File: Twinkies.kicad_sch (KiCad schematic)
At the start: 0 parts

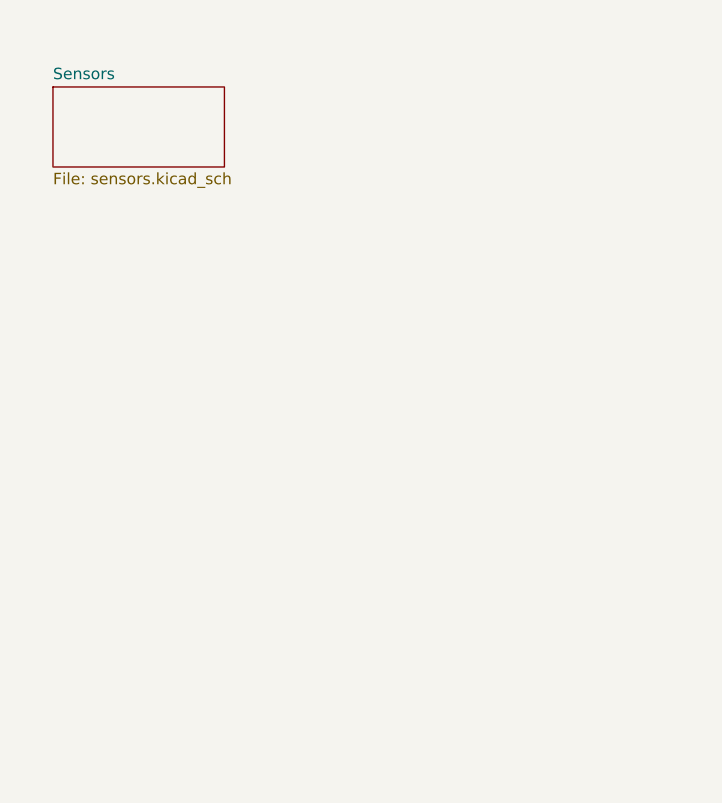
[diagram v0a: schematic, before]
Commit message: 3.4
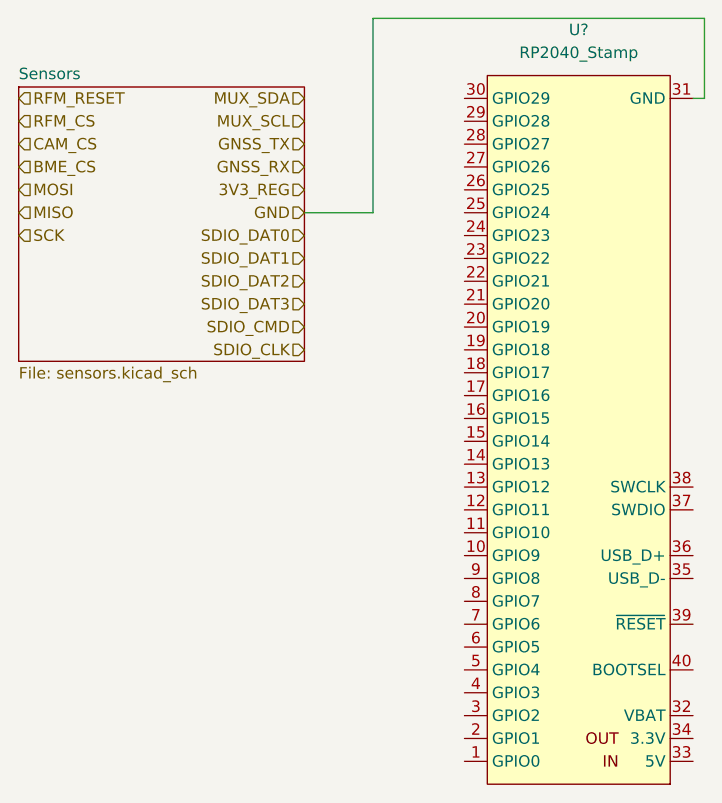
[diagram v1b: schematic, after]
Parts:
- added U?: RP2040_Stamp, RP2040_Stamp:RP2040_Stamp_SMD, symbol RP2040_Stamp:RP2040_Stamp
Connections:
- new net GND: U?.31 (GND)

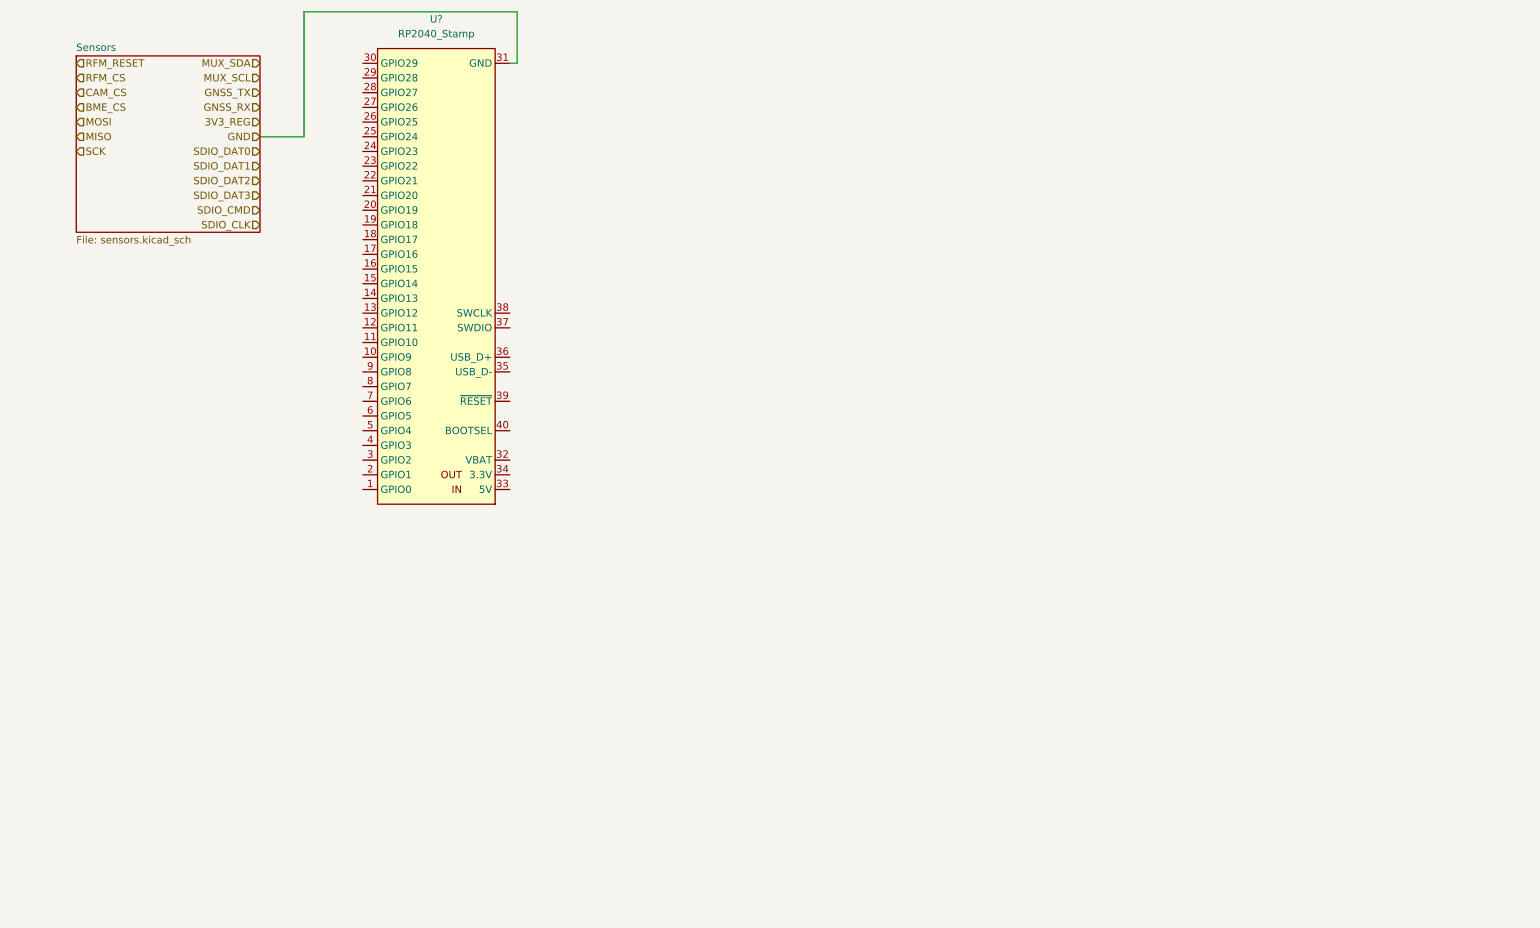
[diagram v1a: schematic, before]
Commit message: 3/6
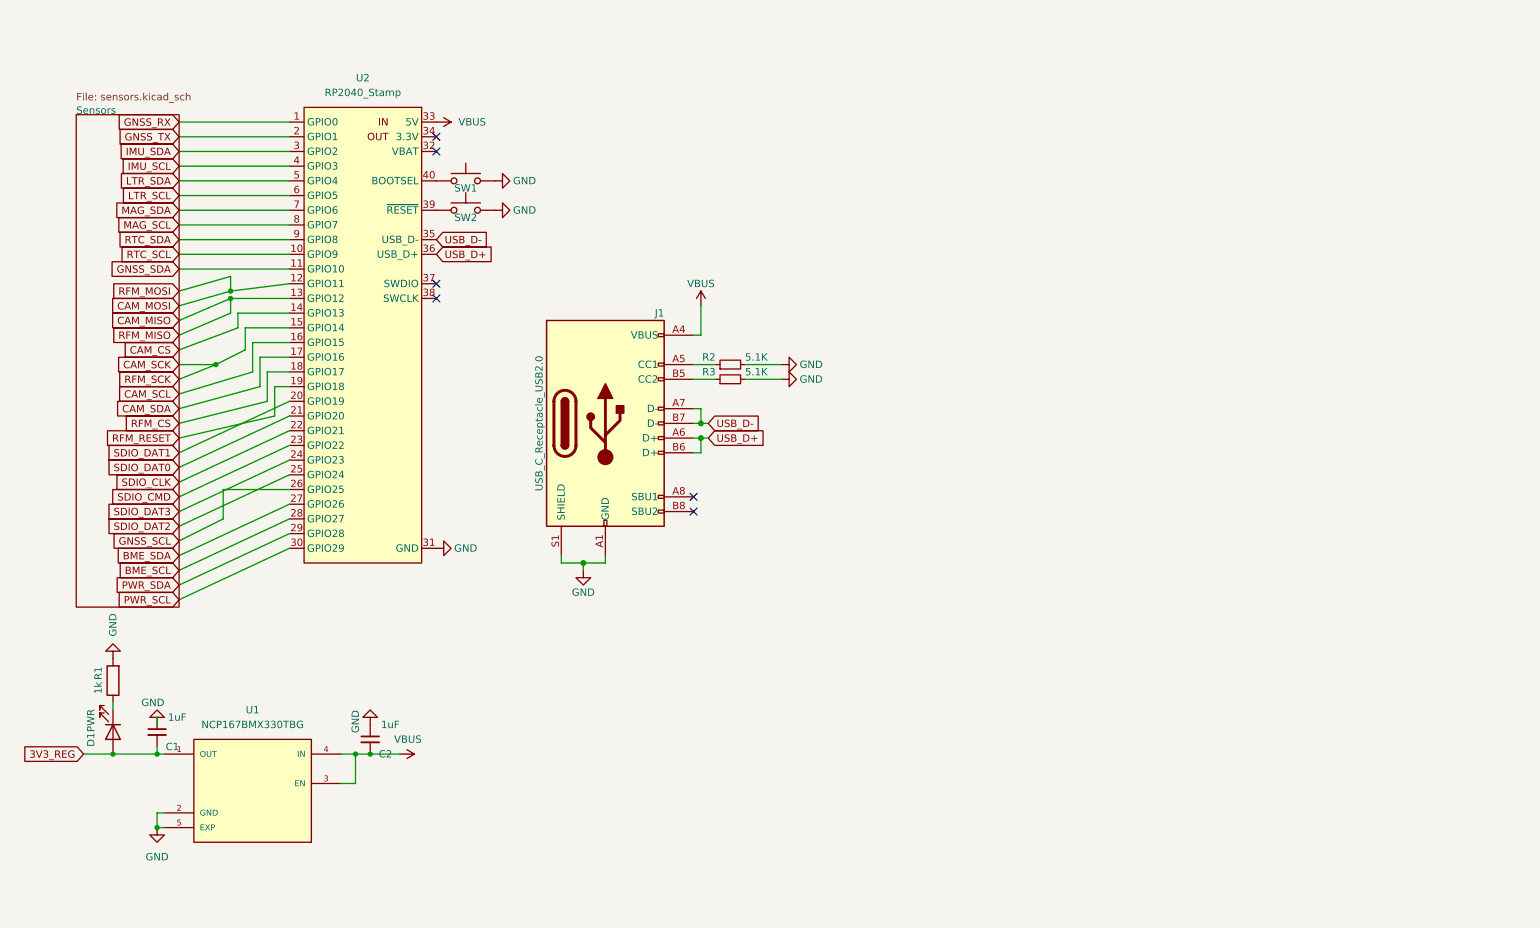
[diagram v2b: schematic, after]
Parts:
- added C1, C2: 1uF, Capacitor_SMD:C_0603_1608Metric, symbol Device:C_Small
- added D1: PWR, LED_SMD:LED_0603_1608Metric, symbol Device:LED
- added J1: USB_C_Receptacle_USB2.0, Connector_USB:USB_C_Receptacle_XKB_U262-16XN-4BVC11, symbol Connector:USB_C_Receptacle_USB2.0
- added R1: 1k, Resistor_SMD:R_0603_1608Metric, symbol Device:R
- added R2, R3: 5.1K, Resistor_SMD:R_0603_1608Metric, symbol Device:R_Small
- added SW1, SW2: RESET, Button_Switch_SMD:SW_Push_SPST_NO_Alps_SKRK, symbol Switch:SW_Push
- added U1: NCP167BMX330TBG, REG_NCP167BMX330TBG, symbol NCP167BMX330TBG:NCP167BMX330TBG
- gave numbers to parts that had none: 1
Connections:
- net 3V3_REG: now also C1.2, D1.2 (A), U1.1 (OUT)
- net CAM_CS: now also U2.14 (GPIO13)
- net GND: now also C1.1, C2.1, J1.A1 (GND), J1.A12 (GND), J1.B1 (GND), J1.B12 (GND), J1.S1 (SHIELD), R1.2, R2.2, R3.2, SW1.2, SW2.2, U1.2 (GND), U1.5 (EXP)
- net GNSS_RX: now also U2.1 (GPIO0)
- net GNSS_TX: now also U2.2 (GPIO1)
- net RFM_CS: now also U2.18 (GPIO17)
- net RFM_RESET: now also U2.19 (GPIO18)
- net SDIO_CLK: now also U2.22 (GPIO21)
- net SDIO_CMD: now also U2.23 (GPIO22)
- net SDIO_DAT0: now also U2.21 (GPIO20)
- net SDIO_DAT1: now also U2.20 (GPIO19)
- net SDIO_DAT2: now also U2.25 (GPIO24)
- net SDIO_DAT3: now also U2.24 (GPIO23)
- net RTC_SCL: now reaches U2.10 (GPIO9)
- net GNSS_SDA: now reaches U2.11 (GPIO10)
- net CAM_MOSI: now reaches U2.12 (GPIO11)
- net CAM_MISO: now reaches U2.13 (GPIO12)
- net CAM_SCK: now reaches U2.15 (GPIO14)
- net CAM_SCL: now reaches U2.16 (GPIO15)
- net CAM_SDA: now reaches U2.17 (GPIO16)
- net GNSS_SCL: now reaches U2.26 (GPIO25)
- net BME_SDA: now reaches U2.27 (GPIO26)
- net BME_SCL: now reaches U2.28 (GPIO27)
- net PWR_SDA: now reaches U2.29 (GPIO28)
- net IMU_SDA: now reaches U2.3 (GPIO2)
- net PWR_SCL: now reaches U2.30 (GPIO29)
- net VBUS: now reaches U2.33 (5V)
- net VBUS: now also C2.2, J1.A4 (VBUS), J1.A9 (VBUS), J1.B4 (VBUS), J1.B9 (VBUS), U1.3 (EN), U1.4 (IN)
- net USB_D-: now reaches U2.35 (USB_D-)
- net USB_D-: now also J1.A7 (D-), J1.B7 (D-)
- net USB_D+: now reaches U2.36 (USB_D+)
- net USB_D+: now also J1.A6 (D+), J1.B6 (D+)
- net at U2.39 (~{RESET}): now also SW2.1
- net IMU_SCL: now reaches U2.4 (GPIO3)
- net at U2.40 (BOOTSEL): now also SW1.1
- net LTR_SDA: now reaches U2.5 (GPIO4)
- net LTR_SCL: now reaches U2.6 (GPIO5)
- net MAG_SDA: now reaches U2.7 (GPIO6)
- net MAG_SCL: now reaches U2.8 (GPIO7)
- net RTC_SDA: now reaches U2.9 (GPIO8)
- new net: J1.B5 (CC2), R3.1
- new net: J1.A5 (CC1), R2.1
- new net: D1.1 (K), R1.1
- no-connect marks 0 -> 6
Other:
- title: Sensor Board -> RP2040 Stamp
- moved on the sheet: U2

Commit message: pdu design
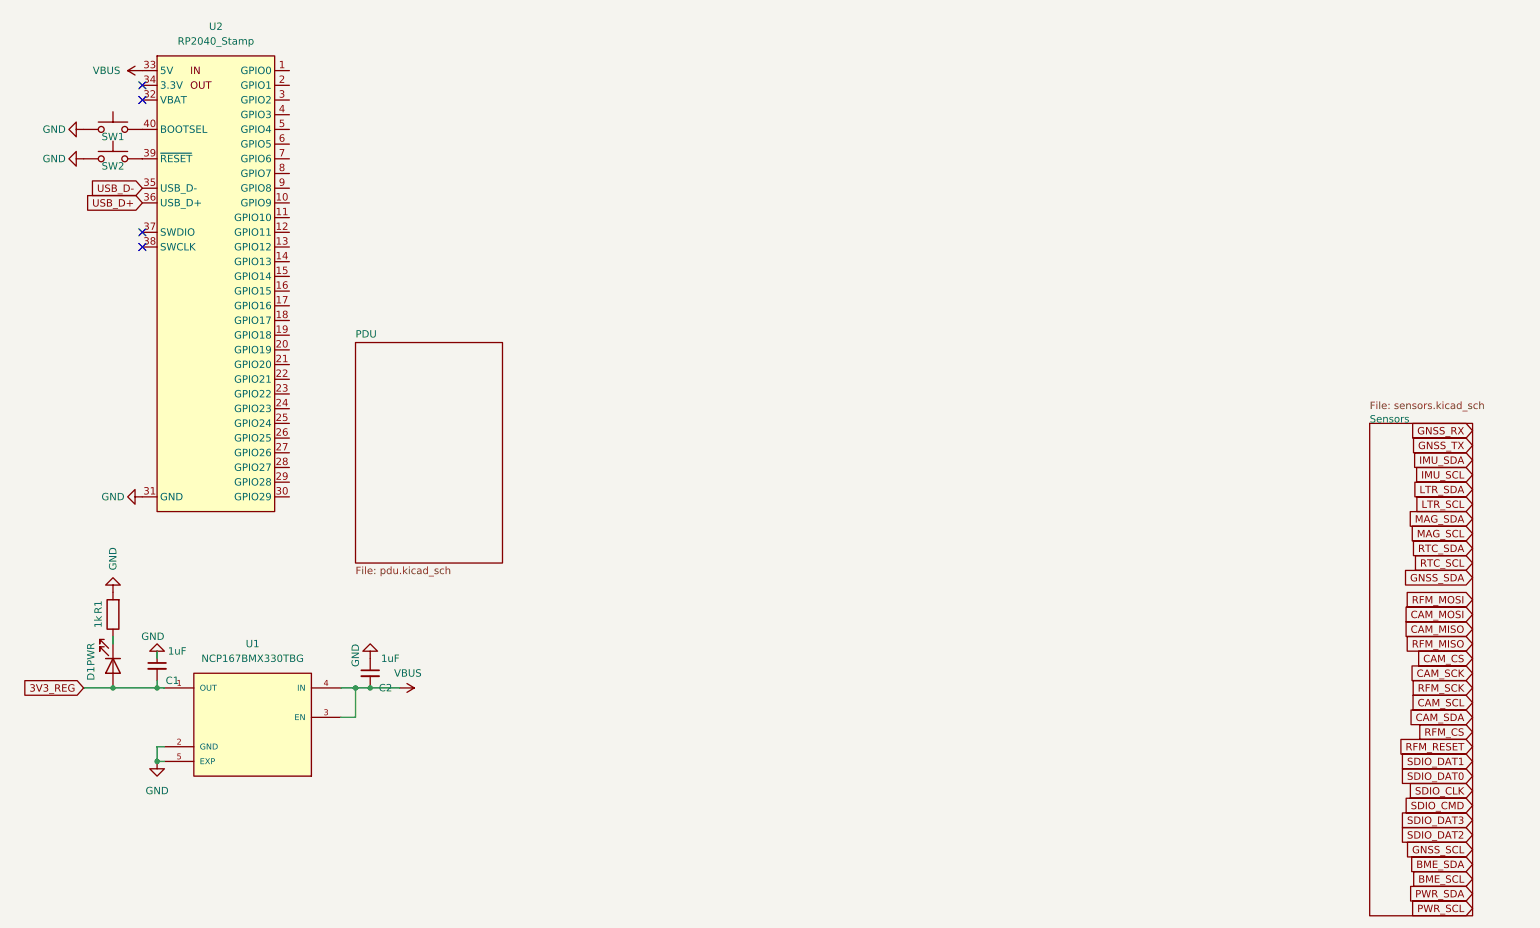
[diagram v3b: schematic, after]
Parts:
- removed J1: USB_C_Receptacle_USB2.0, Connector_USB:USB_C_Receptacle_XKB_U262-16XN-4BVC11, symbol Connector:USB_C_Receptacle_USB2.0
- removed R2, R3: 5.1K, Resistor_SMD:R_0603_1608Metric, symbol Device:R_Small
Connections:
- net BME_SCL: no longer U2.28 (GPIO27)
- net BME_SDA: no longer U2.27 (GPIO26)
- net CAM_CS: no longer U2.14 (GPIO13)
- net CAM_MISO: no longer U2.13 (GPIO12)
- net CAM_MOSI: no longer U2.12 (GPIO11)
- net CAM_SCK: no longer U2.15 (GPIO14)
- net CAM_SCL: no longer U2.16 (GPIO15)
- net CAM_SDA: no longer U2.17 (GPIO16)
- net GNSS_RX: no longer U2.1 (GPIO0)
- net GNSS_SCL: no longer U2.26 (GPIO25)
- net GNSS_SDA: no longer U2.11 (GPIO10)
- net GNSS_TX: no longer U2.2 (GPIO1)
- net IMU_SCL: no longer U2.4 (GPIO3)
- net IMU_SDA: no longer U2.3 (GPIO2)
- net LTR_SCL: no longer U2.6 (GPIO5)
- net LTR_SDA: no longer U2.5 (GPIO4)
- net MAG_SCL: no longer U2.8 (GPIO7)
- net MAG_SDA: no longer U2.7 (GPIO6)
- net PWR_SCL: no longer U2.30 (GPIO29)
- net PWR_SDA: no longer U2.29 (GPIO28)
- net RFM_CS: no longer U2.18 (GPIO17)
- net RFM_RESET: no longer U2.19 (GPIO18)
- net RTC_SCL: no longer U2.10 (GPIO9)
- net RTC_SDA: no longer U2.9 (GPIO8)
- net SDIO_CLK: no longer U2.22 (GPIO21)
- net SDIO_CMD: no longer U2.23 (GPIO22)
- net SDIO_DAT0: no longer U2.21 (GPIO20)
- net SDIO_DAT1: no longer U2.20 (GPIO19)
- net SDIO_DAT2: no longer U2.25 (GPIO24)
- net SDIO_DAT3: no longer U2.24 (GPIO23)
- no-connect marks 6 -> 4
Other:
- added sheet PDU (pdu.kicad_sch)
- moved on the sheet: C1, C2, D1, R1, SW1, SW2, U1, U2

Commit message: Apr 8
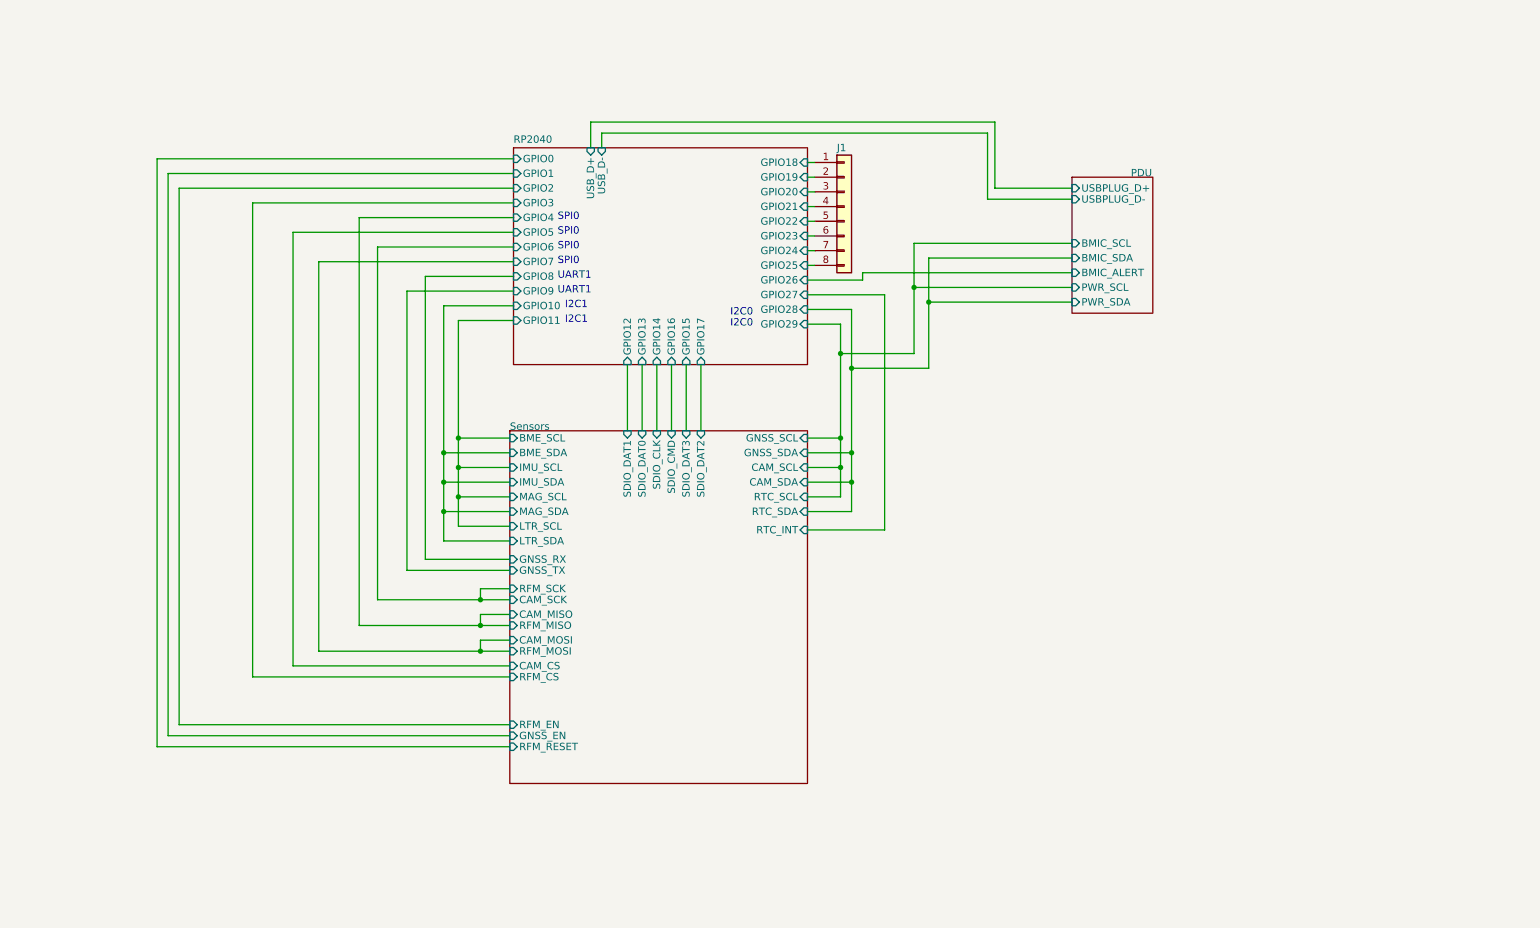
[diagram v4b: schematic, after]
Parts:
- removed C1, C2: 1uF, Capacitor_SMD:C_0603_1608Metric, symbol Device:C_Small
- removed D1: PWR, LED_SMD:LED_0603_1608Metric, symbol Device:LED
- removed R1: 1k, Resistor_SMD:R_0603_1608Metric, symbol Device:R
- removed SW1, SW2: RESET, Button_Switch_SMD:SW_Push_SPST_NO_Alps_SKRK, symbol Switch:SW_Push
- removed U1: NCP167BMX330TBG, REG_NCP167BMX330TBG, symbol NCP167BMX330TBG:NCP167BMX330TBG
- removed U2: RP2040_Stamp, RP2040_Stamp:RP2040_Stamp_SMD, symbol RP2040_Stamp:RP2040_Stamp
- added J1: Conn_01x08, Connector_PinHeader_2.00mm:PinHeader_1x08_P2.00mm_Vertical, symbol Connector_Generic:Conn_01x08
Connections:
- new net RP2040/GPIO18: J1.1 (Pin_1)
- new net RP2040/GPIO19: J1.2 (Pin_2)
- new net RP2040/GPIO20: J1.3 (Pin_3)
- new net RP2040/GPIO21: J1.4 (Pin_4)
- new net RP2040/GPIO22: J1.5 (Pin_5)
- new net RP2040/GPIO23: J1.6 (Pin_6)
- new net RP2040/GPIO24: J1.7 (Pin_7)
- new net RP2040/GPIO25: J1.8 (Pin_8)
- no-connect marks 4 -> 0
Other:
- added sheet RP2040 (rp2040.kicad_sch)
- sheet PDU ports: added BMIC_ALERT, BMIC_SCL, BMIC_SDA, PWR_SCL, PWR_SDA, USBPLUG_D+, USBPLUG_D-; removed none
- sheet Sensors ports: added BME_SCL, BME_SDA, CAM_CS, CAM_MISO, CAM_MOSI, CAM_SCK, CAM_SCL, CAM_SDA, GNSS_EN, GNSS_RX, GNSS_SCL, GNSS_SDA, GNSS_TX, IMU_SCL, IMU_SDA, LTR_SCL, LTR_SDA, MAG_SCL, MAG_SDA, RFM_CS, RFM_EN, RFM_MISO, RFM_MOSI, RFM_RESET, RFM_SCK, RTC_INT, RTC_SCL, RTC_SDA, SDIO_CLK, SDIO_CMD, SDIO_DAT0, SDIO_DAT1, SDIO_DAT2, SDIO_DAT3; removed none
- note added: "I2C0"
- note added: "I2C1"
- note added: "SPI0"
- note added: "UART1"
